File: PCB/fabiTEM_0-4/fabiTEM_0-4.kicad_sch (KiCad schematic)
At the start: 80 parts, among them J1 MJ-4PP-9, J2 MJ-4PP-9, U1 xiao-rp2040, U2 xiao-rp2040

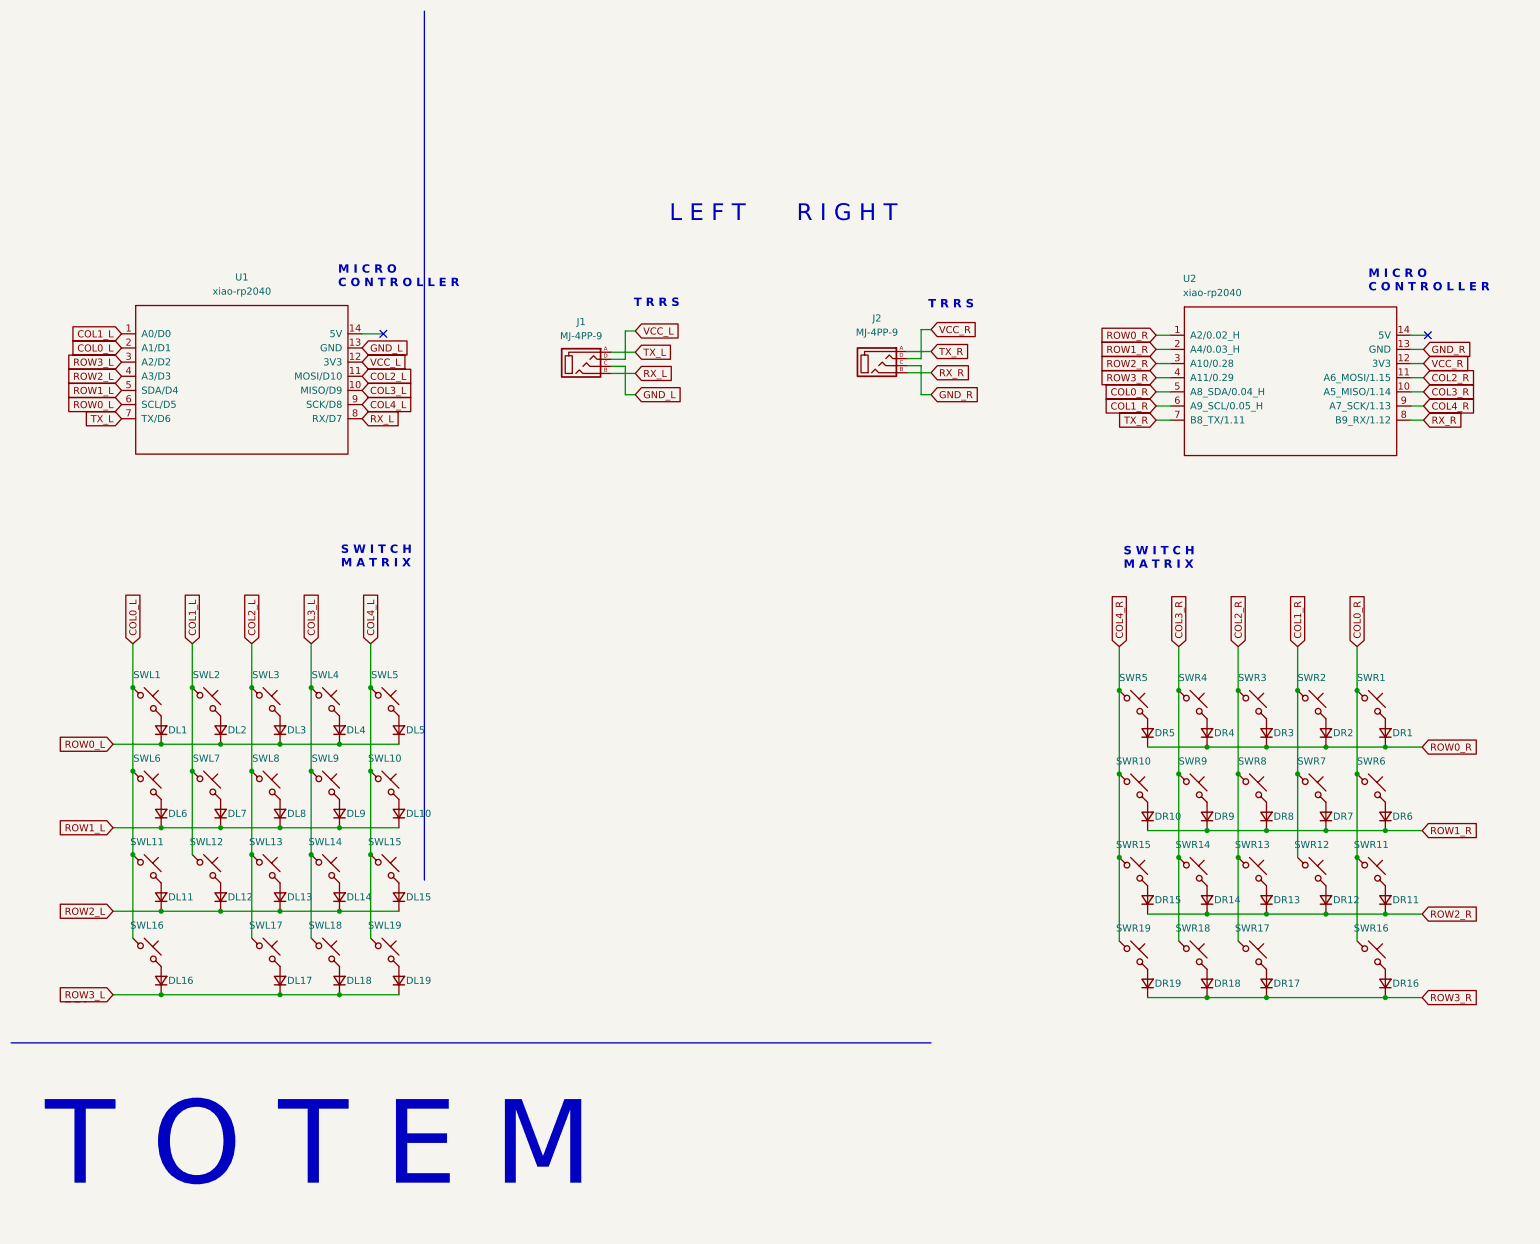
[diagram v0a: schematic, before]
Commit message: v0.5
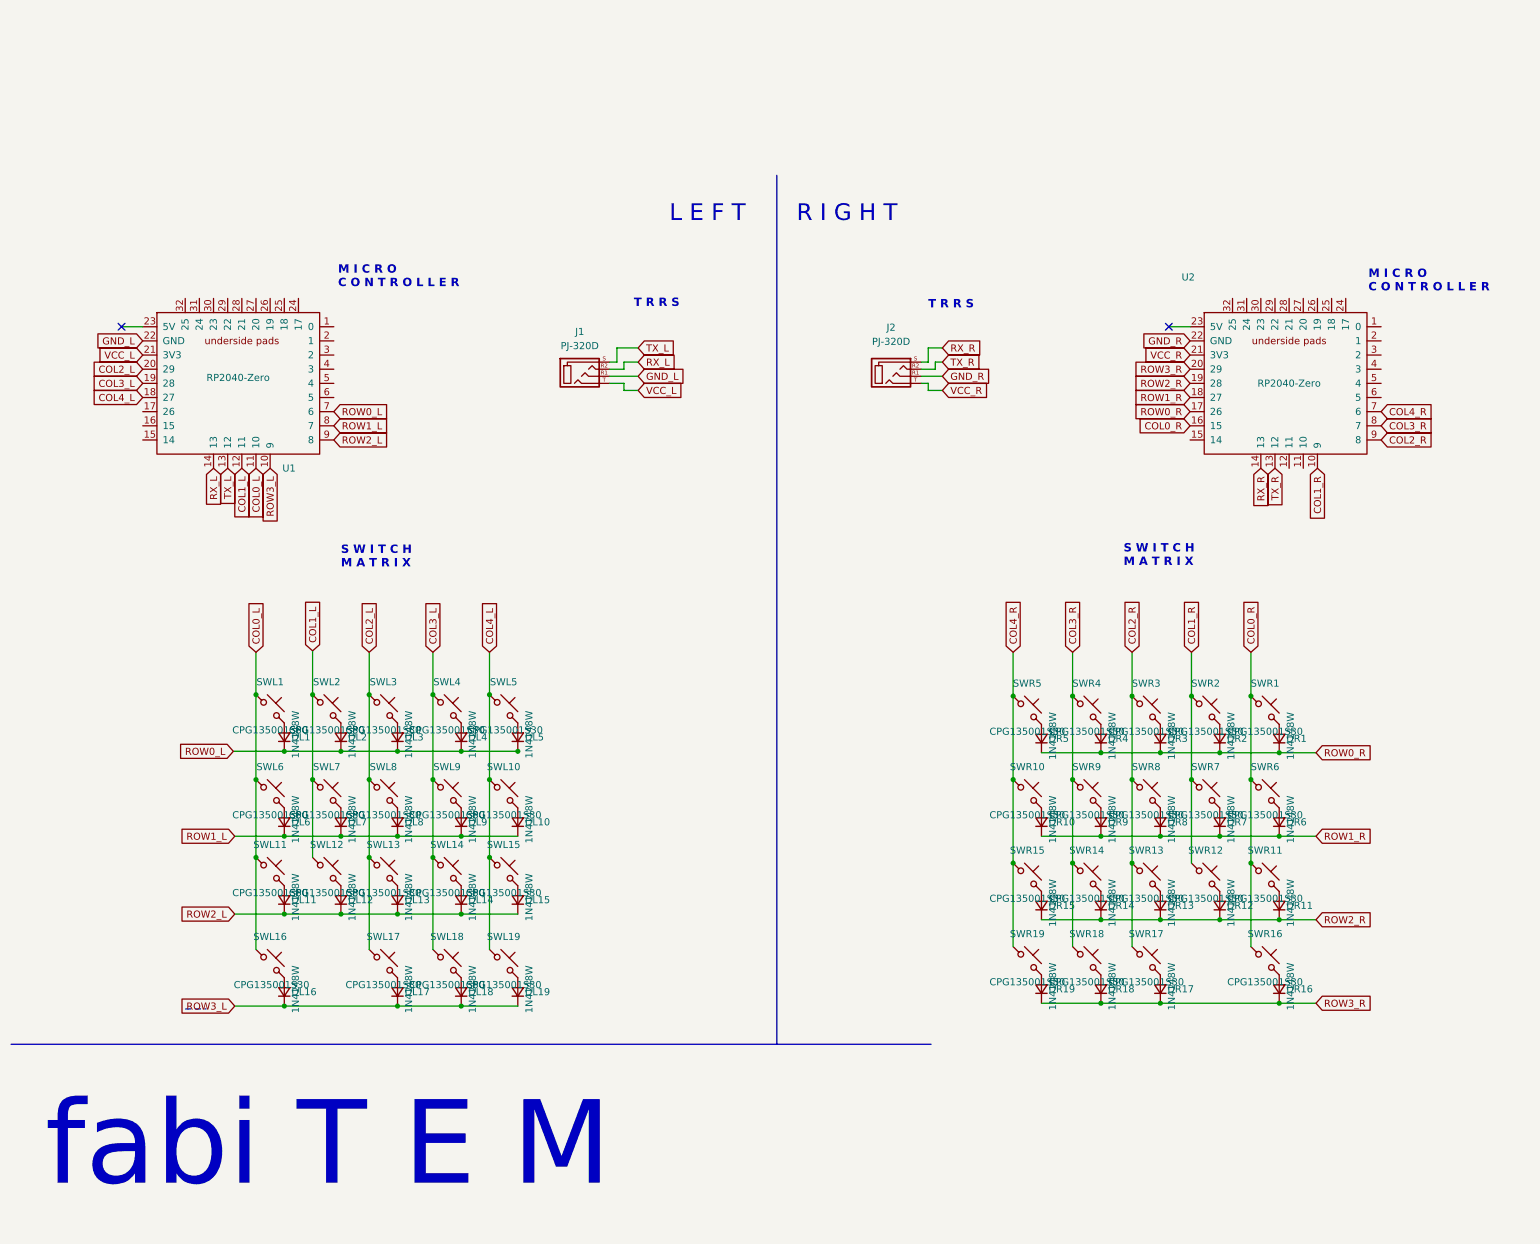
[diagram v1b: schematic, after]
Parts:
- DL1, DL10, DL11, DL12, DL13, DL14, DL15, DL16, DL17, DL18, DL19, DL2, DL3, DL4, DL5, DL6, DL7, DL8, DL9, DR1, DR10, DR11, DR12, DR13, DR14, DR15, DR16, DR17, DR18, DR19, DR2, DR3, DR4, DR5, DR6, DR7, DR8, DR9: value D_Small -> 1N4148W; footprint TOTEMlib:Diode_SOD123 -> fabiTEM:Diode_SOD123; symbol Device:D_Small -> fabiTEM:D_Small
- J1: value MJ-4PP-9 -> PJ-320D; footprint TOTEMlib:MJ-4PP-9_1side -> Connector_Audio:Jack_3.5mm_PJ320D_Horizontal
- J2: value MJ-4PP-9 -> PJ-320D; footprint TOTEMlib:MJ-4PP-9_1side -> Connector_Audio:Jack_3.5mm_PJ320D_Horizontal; symbol kbd:MJ-4PP-9 -> fabiTEM:PJ320D
- SWL1, SWL10, SWL11, SWL12, SWL13, SWL14, SWL15, SWL16, SWL17, SWL18, SWL19, SWL2, SWL3, SWL4, SWL5, SWL6, SWL7, SWL8, SWL9, SWR1, SWR10, SWR11, SWR12, SWR13, SWR14, SWR15, SWR16, SWR17, SWR18, SWR19, SWR2, SWR3, SWR4, SWR5, SWR6, SWR7, SWR8, SWR9: value SW_Push_45deg -> CPG135001S30; footprint TOTEMlib:Kailh_socket_PG1350_optional -> fabiTEM:Kailh_socket_PG1350_reverse; symbol Switch:SW_Push_45deg -> fabiTEM:SW_Push_45deg
- U1, U2: value xiao-rp2040 -> RP2040-Zero; footprint XIAO_PCB:xiao RP2040 MOUDLE14P-2.54-21X17.8MM -> mcu:rp2040-zero-smd-pads; symbol xiaoRP2040:xiao-rp2040 -> mcu:rp2040-zero-pads
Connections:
- net COL0_L: now also U1.11 (10); no longer U1.2 (A1/D1)
- net COL0_R: now also U2.16 (15); no longer U2.5 (A8_SDA/0.04_H)
- net COL1_L: now also U1.12 (11); no longer U1.1 (A0/D0)
- net COL1_R: now also U2.10 (9); no longer U2.6 (A9_SCL/0.05_H)
- net COL2_L: now also U1.20 (29); no longer U1.11 (MOSI/D10)
- net COL2_R: now also U2.9 (8); no longer U2.11 (A6_MOSI/1.15)
- net COL3_L: now also U1.19 (28); no longer U1.10 (MISO/D9)
- net COL3_R: now also U2.8 (7); no longer U2.10 (A5_MISO/1.14)
- net COL4_L: now also U1.18 (27); no longer U1.9 (SCK/D8)
- net COL4_R: now also U2.7 (6); no longer U2.9 (A7_SCK/1.13)
- net GND_L: now also J1.R1, U1.22 (GND), U1.33 (GND); no longer J1.C, U1.13 (GND)
- net GND_R: now also J2.R1, U2.22 (GND), U2.33 (GND); no longer J2.C, U2.13 (GND)
- net ROW0_L: now also U1.7 (6); no longer U1.6 (SCL/D5)
- net ROW0_R: now also U2.17 (26); no longer U2.1 (A2/0.02_H)
- net ROW1_L: now also U1.8 (7); no longer U1.5 (SDA/D4)
- net ROW1_R: now also U2.18 (27); no longer U2.2 (A4/0.03_H)
- net ROW2_L: now also U1.9 (8); no longer U1.4 (A3/D3)
- net ROW2_R: now also U2.19 (28); no longer U2.3 (A10/0.28)
- net ROW3_L: now also U1.10 (9); no longer U1.3 (A2/D2)
- net ROW3_R: now also U2.20 (29); no longer U2.4 (A11/0.29)
- net RX_L: now also J1.R2, U1.14 (13); no longer J1.B, U1.8 (RX/D7)
- net RX_R: now also J2.S, U2.14 (13); no longer J2.B, U2.8 (B9_RX/1.12)
- net TX_L: now also J1.S, U1.13 (12); no longer J1.A, U1.7 (TX/D6)
- net TX_R: now also J2.R2, U2.13 (12); no longer J2.A, U2.7 (B8_TX/1.11)
- net VCC_L: now also J1.T, U1.21 (3V3); no longer J1.D, U1.12 (3V3)
- net VCC_R: now also J2.T, U2.21 (3V3); no longer J2.D, U2.12 (3V3)
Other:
- note added: "fabi T E M"
- note removed: "T O T E M"
- title: TOTEM split keyboard -> fabiTEM split keyboard
- moved on the sheet: DL1, DL10, DL11, DL12, DL13, DL14, DL15, DL16, DL17, DL18, DL19, DL2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
